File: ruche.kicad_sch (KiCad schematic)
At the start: 30 parts, among them IC2 MAX17048G+, IC3 L86-M33, IC4 SHT41-AD1B-R3, J13 Micro_SD_Card, U1 MKRWAN_1310, U2 MS5611-01BA, U3 XC6220B331MR

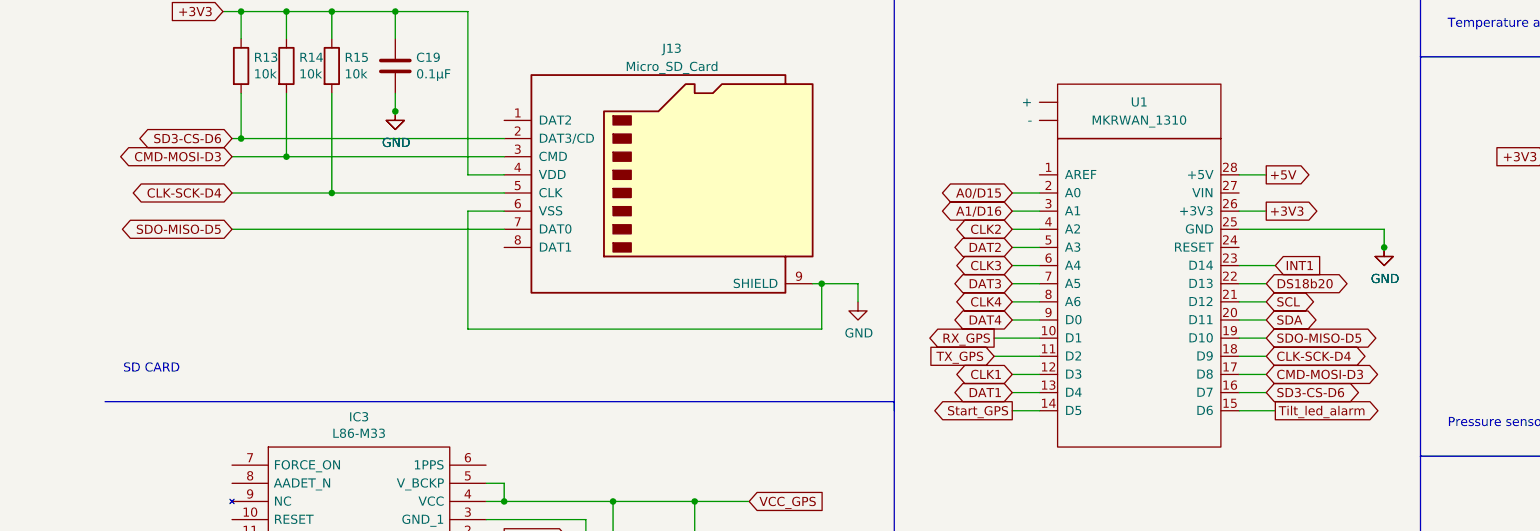
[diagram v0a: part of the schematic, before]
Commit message: Modification routage
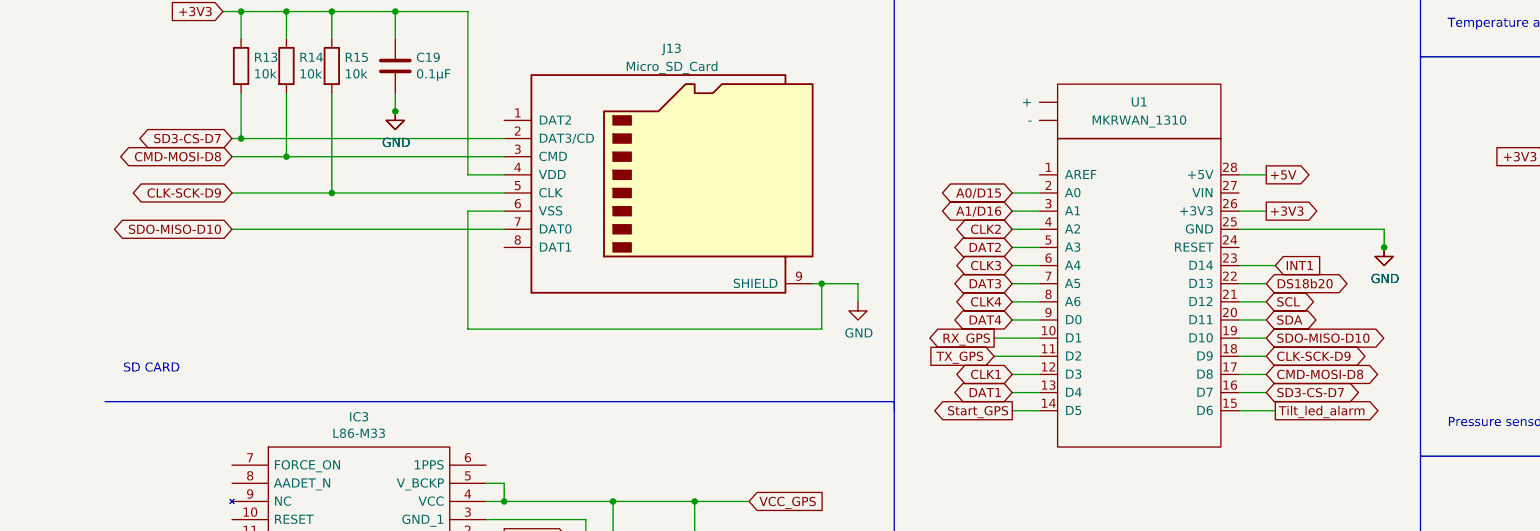
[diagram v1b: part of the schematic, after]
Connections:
- net CLK-SCK-D4 renamed CLK-SCK-D9
- net CMD-MOSI-D3 renamed CMD-MOSI-D8
- net SD3-CS-D6 renamed SD3-CS-D7
- net SDO-MISO-D5 renamed SDO-MISO-D10
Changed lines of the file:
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@@
     )
   )
-  (global_label "SD3-CS-D6" (shape bidirectional) (at 175.26 111.76 0) (fields_autoplaced)
+  (global_label "SD3-CS-D7" (shape bidirectional) (at 175.26 111.76 0) (fields_autoplaced)
     (effects (font (size 1.27 1.27)) (justify left))
     (property "Intersheet References" "${INTERSHEET_REFS}" (id 0) (at 189.3771 111.6806 0)
@@
     )
   )
-  (global_label "SD3-CS-D6" (shape bidirectional) (at 30.48 76.2 180) (fields_autoplaced)
+  (global_label "SD3-CS-D7" (shape bidirectional) (at 30.48 76.2 180) (fields_autoplaced)
     (effects (font (size 1.27 1.27)) (justify right))
     (property "Intersheet References" "${INTERSHEET_REFS}" (id 0) (at 16.3629 76.1206 0)
@@
     )
   )
-  (global_label "CLK-SCK-D4" (shape bidirectional) (at 30.48 83.82 180) (fields_autoplaced)
+  (global_label "CLK-SCK-D9" (shape bidirectional) (at 30.48 83.82 180) (fields_autoplaced)
     (effects (font (size 1.27 1.27)) (justify right))
     (property "Intersheet References" "${INTERSHEET_REFS}" (id 0) (at 15.2139 83.7406 0)
@@
     )
   )
-  (global_label "SDO-MISO-D5" (shape bidirectional) (at 175.26 104.14 0) (fields_autoplaced)
-    (effects (font (size 1.27 1.27)) (justify left))
-    (property "Intersheet References" "${INTERSHEET_REFS}" (id 0) (at 191.6147 104.0606 0)
+  (global_label "SDO-MISO-D10" (shape bidirectional) (at 175.26 104.14 0) (fields_autoplaced)
+    (effects (font (size 1.27 1.27)) (justify left))
+    (property "Intersheet References" "${INTERSHEET_REFS}" (id 0) (at 192.8242 104.0606 0)
       (effects (font (size 1.27 1.27)) (justify left) hide)
     )
@@
     )
   )
-  (global_label "CLK-SCK-D4" (shape bidirectional) (at 175.26 106.68 0) (fields_autoplaced)
+  (global_label "CLK-SCK-D9" (shape bidirectional) (at 175.26 106.68 0) (fields_autoplaced)
     (effects (font (size 1.27 1.27)) (justify left))
     (property "Intersheet References" "${INTERSHEET_REFS}" (id 0) (at 190.5261 106.6006 0)
@@
     )
   )
-  (global_label "CMD-MOSI-D3" (shape bidirectional) (at 175.26 109.22 0) (fields_autoplaced)
+  (global_label "CMD-MOSI-D8" (shape bidirectional) (at 175.26 109.22 0) (fields_autoplaced)
     (effects (font (size 1.27 1.27)) (justify left))
     (property "Intersheet References" "${INTERSHEET_REFS}" (id 0) (at 191.7961 109.1406 0)
@@
     )
   )
-  (global_label "CMD-MOSI-D3" (shape bidirectional) (at 30.48 78.74 180) (fields_autoplaced)
+  (global_label "CMD-MOSI-D8" (shape bidirectional) (at 30.48 78.74 180) (fields_autoplaced)
     (effects (font (size 1.27 1.27)) (justify right))
     (property "Intersheet References" "${INTERSHEET_REFS}" (id 0) (at 13.9439 78.6606 0)
@@
     )
   )
-  (global_label "SDO-MISO-D5" (shape bidirectional) (at 30.48 88.9 180) (fields_autoplaced)
-    (effects (font (size 1.27 1.27)) (justify right))
-    (property "Intersheet References" "${INTERSHEET_REFS}" (id 0) (at 14.1253 88.8206 0)
-      (effects (font (size 1.27 1.27)) (justify right) hide)
-    )
+  (global_label "SDO-MISO-D10" (shape bidirectional) (at 30.48 88.9 180) (fields_autoplaced)
+    (effects (font (size 1.27 1.27)) (justify right))
+    (property "Intersheet References" "${INTERSHEET_REFS}" (id 0) (at 12.9158 88.8206 0)
+      (effects (font (size 1.27 1.27)) (justify right) hide)
+    )
